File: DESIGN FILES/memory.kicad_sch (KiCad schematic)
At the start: 20 parts, among them J601 TF-15x15, U601 IS42S16160J-6BLI, U602 IS25WP064A-JBLE

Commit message: changes and adding schematic pdf
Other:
- company: Soundsom -> Joël Ucedo
- title: Memory -> MIMXRT1064 MCU Module
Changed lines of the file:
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@@
   (paper "A3")
   (title_block
-    (title "Memory")
-    (date "2023-05-19")
+    (title "MIMXRT1064 MCU Module")
+    (date "2023-05-23")
     (rev "0")
-    (company "Soundsom")
+    (company "Joël Ucedo")
   )
   (junction (at 288.29 102.87) (diameter 0) (color 0 0 0 0)

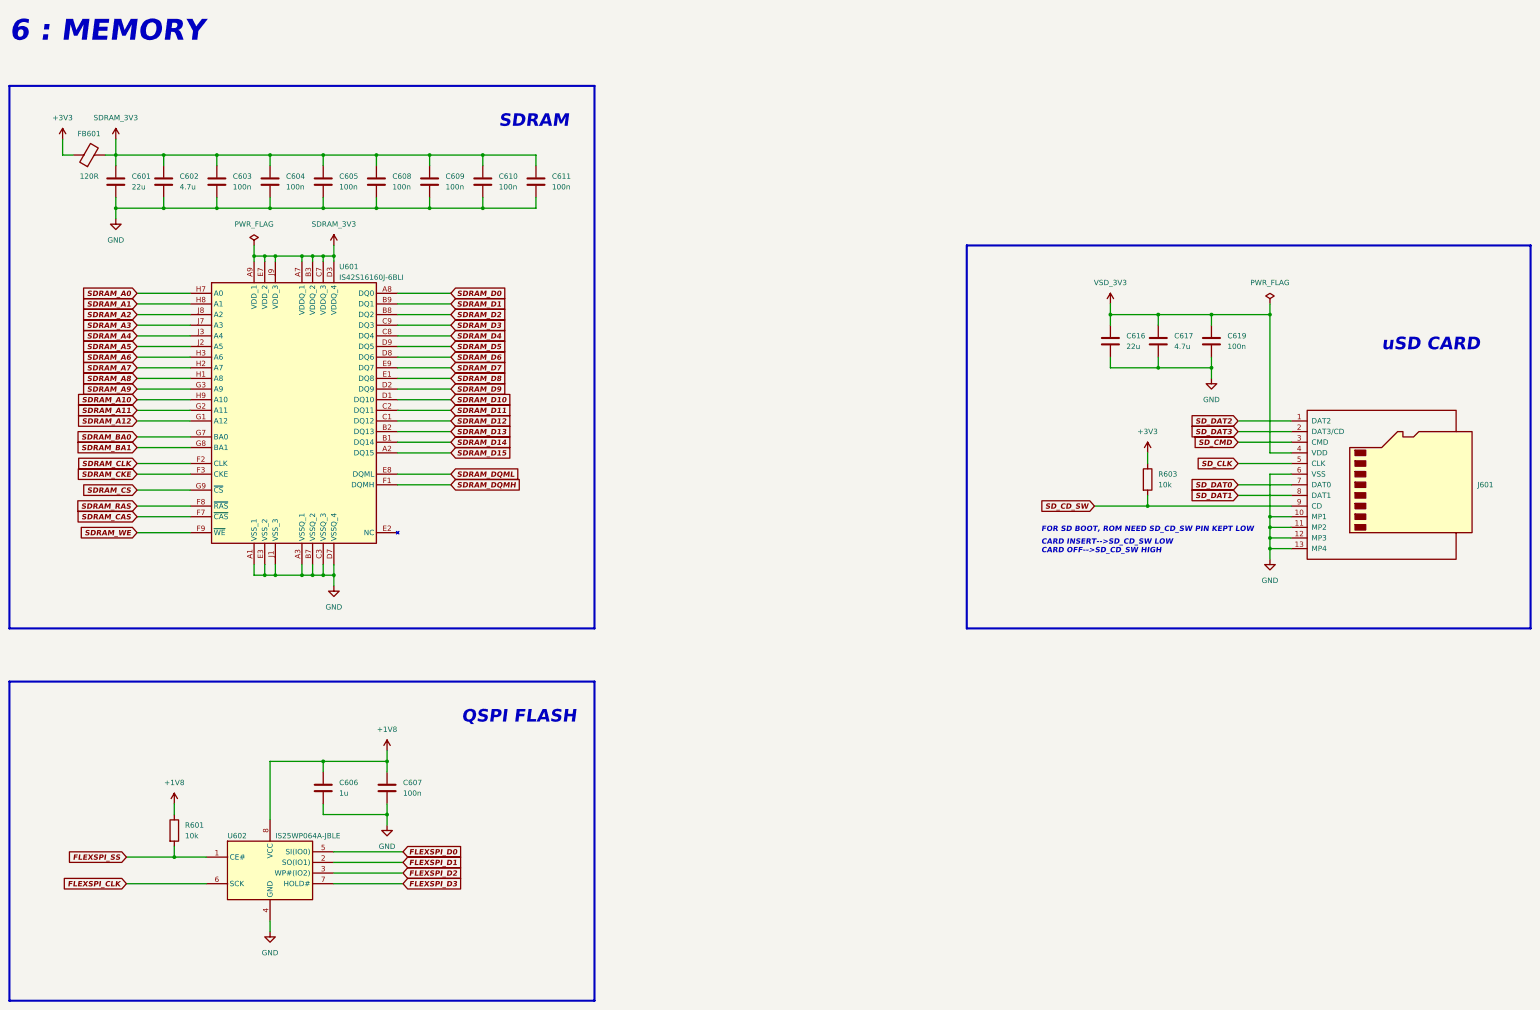
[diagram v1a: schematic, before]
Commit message: updates
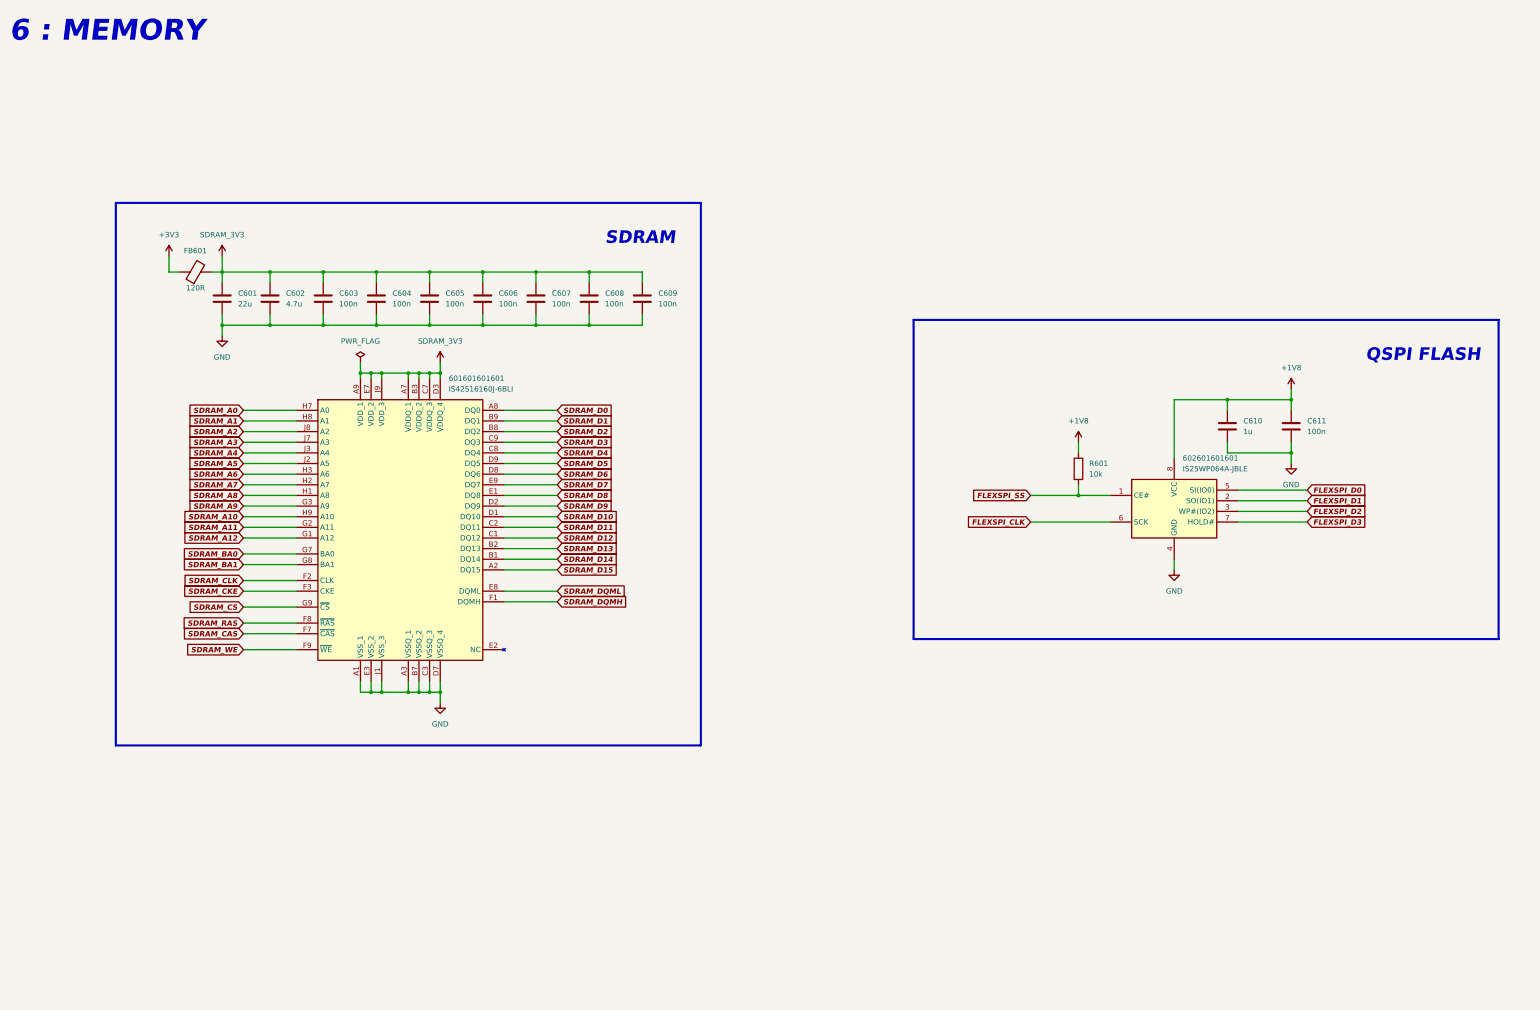
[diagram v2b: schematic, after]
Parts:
- removed C601, C616: 22u, MIMXRT1064 MCU Module:0603_CL10A226MQ8NRNC, symbol MIMXRT1064 MCU Module:CL10A226MQ8NRNC
- removed C602, C617: 4.7u, MIMXRT1064 MCU Module:0402_CL05A475MP5NRNC, symbol MIMXRT1064 MCU Module:CL05A475MP5NRNC
- removed C603, C604, C605, C607, C608, C609, C610, C611, C619: 100n, MIMXRT1064 MCU Module:0402_CL05B104KB54PNC, symbol MIMXRT1064 MCU Module:CL05B104KB54PNC
- removed C606: 1u, MIMXRT1064 MCU Module:0402_CL05A105KA5NQNC, symbol MIMXRT1064 MCU Module:CL05A105KA5NQNC
- removed FB601: 120R, MIMXRT1064 MCU Module:0603_BLM18AG121SN1D, symbol MIMXRT1064 MCU Module:BLM18AG121SN1D
- removed J601: TF-15x15, MIMXRT1064 MCU Module:TF-15x15_smd, symbol MIMXRT1064 MCU Module:TF-15x15
- removed R601, R603: 10k, MIMXRT1064 MCU Module:0402WGF1002TCE, symbol MIMXRT1064 MCU Module:0402WGF1002TCE
- removed U601: IS42S16160J-6BLI, MIMXRT1064 MCU Module:IS42S16160J-6BLI, symbol MIMXRT1064 MCU Module:IS42S16160J-6BLI
- removed U602: IS25WP064A-JBLE, MIMXRT1064 MCU Module:IS25WP064A-JBLE, symbol MIMXRT1064 MCU Module:IS25WP064A-JBLE
- added 601601601601: IS42S16160J-6BLI, MY MEMORY AND STORAGE LIBRARY:IS42S16160J-6BLI, symbol MY MEMORY AND STORAGE LIBRARY:IS42S16160J-6BLI
- added 602601601601: IS25WP064A-JBLE, MY MEMORY AND STORAGE LIBRARY:IS25WP064A-JBLE, symbol MY MEMORY AND STORAGE LIBRARY:IS25WP064A-JBLE
- added C601: 22u, MY CAPACITOR LIBRARY:0603_CL10A226MQ8NRNC, symbol MY CAPACITOR LIBRARY:CL10A226MQ8NRNC
- added C602: 4.7u, MY CAPACITOR LIBRARY:0402_CL05A475MP5NRNC, symbol MY CAPACITOR LIBRARY:CL05A475MP5NRNC
- added C603, C604, C605, C606, C607, C608, C609, C611: 100n, MY CAPACITOR LIBRARY:0402_CL05B104KB54PNC, symbol MY CAPACITOR LIBRARY:CL05B104KB54PNC
- added C610: 1u, MY CAPACITOR LIBRARY:0402_CL05A105KA5NQNC, symbol MY CAPACITOR LIBRARY:CL05A105KA5NQNC
- added FB601: 120R, MY FERRITE BEAD LIBRARY:0603_BLM18AG121SN1D, symbol MY FERRITE BEAD LIBRARY:BLM18AG121SN1D
- added R601: 10k, MY RESISTOR LIBRARY:0402WGF1002TCE, symbol MY RESISTOR LIBRARY:0402WGF1002TCE
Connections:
- net +1V8: now also 602601601601.8 (VCC), C610.1, C611.1, R601.1
- net +3V3: now also FB601.1
- net FLEXSPI_CLK: now also 602601601601.6 (SCK)
- net FLEXSPI_D0: now also 602601601601.5 (SI(IO0))
- net FLEXSPI_D1: now also 602601601601.2 (SO(IO1))
- net FLEXSPI_D2: now also 602601601601.3 (WP#(IO2))
- net FLEXSPI_D3: now also 602601601601.7 (HOLD#)
- net FLEXSPI_SS: now also 602601601601.1 (CE#), R601.2
- net GND: now also 601601601601.A1 (VSS_1), 601601601601.A3 (VSSQ_1), 601601601601.B7 (VSSQ_2), 601601601601.C3 (VSSQ_3), 601601601601.D7 (VSSQ_4), 601601601601.E3 (VSS_2), 601601601601.J1 (VSS_3), 602601601601.4 (GND), C601.2, C602.2, C603.2, C604.2, C605.2, C606.2, C607.2, C608.2, C609.2, C610.2, C611.2
- net SDRAM_3V3: now also 601601601601.A7 (VDDQ_1), 601601601601.A9 (VDD_1), 601601601601.B3 (VDDQ_2), 601601601601.C7 (VDDQ_3), 601601601601.D3 (VDDQ_4), 601601601601.E7 (VDD_2), 601601601601.J9 (VDD_3), C601.1, C602.1, C603.1, C604.1, C605.1, C606.1, C607.1, C608.1, C609.1, FB601.2
- net SDRAM_A0: now also 601601601601.H7 (A0)
- net SDRAM_A1: now also 601601601601.H8 (A1)
- net SDRAM_A10: now also 601601601601.H9 (A10)
- net SDRAM_A11: now also 601601601601.G2 (A11)
- net SDRAM_A12: now also 601601601601.G1 (A12)
- net SDRAM_A2: now also 601601601601.J8 (A2)
- net SDRAM_A3: now also 601601601601.J7 (A3)
- net SDRAM_A4: now also 601601601601.J3 (A4)
- net SDRAM_A5: now also 601601601601.J2 (A5)
- net SDRAM_A6: now also 601601601601.H3 (A6)
- net SDRAM_A7: now also 601601601601.H2 (A7)
- net SDRAM_A8: now also 601601601601.H1 (A8)
- net SDRAM_A9: now also 601601601601.G3 (A9)
- net SDRAM_BA0: now also 601601601601.G7 (BA0)
- net SDRAM_BA1: now also 601601601601.G8 (BA1)
- net SDRAM_CAS: now also 601601601601.F7 (~{CAS})
- net SDRAM_CKE: now also 601601601601.F3 (CKE)
- net SDRAM_CLK: now also 601601601601.F2 (CLK)
- net SDRAM_CS: now also 601601601601.G9 (~{CS})
- net SDRAM_D0: now also 601601601601.A8 (DQ0)
- net SDRAM_D1: now also 601601601601.B9 (DQ1)
- net SDRAM_D10: now also 601601601601.D1 (DQ10)
- net SDRAM_D11: now also 601601601601.C2 (DQ11)
- net SDRAM_D12: now also 601601601601.C1 (DQ12)
- net SDRAM_D13: now also 601601601601.B2 (DQ13)
- net SDRAM_D14: now also 601601601601.B1 (DQ14)
- net SDRAM_D15: now also 601601601601.A2 (DQ15)
- net SDRAM_D2: now also 601601601601.B8 (DQ2)
- net SDRAM_D3: now also 601601601601.C9 (DQ3)
- net SDRAM_D4: now also 601601601601.C8 (DQ4)
- net SDRAM_D5: now also 601601601601.D9 (DQ5)
- net SDRAM_D6: now also 601601601601.D8 (DQ6)
- net SDRAM_D7: now also 601601601601.E9 (DQ7)
- net SDRAM_D8: now also 601601601601.E1 (DQ8)
- net SDRAM_D9: now also 601601601601.D2 (DQ9)
- net SDRAM_DQMH: now also 601601601601.F1 (DQMH)
- net SDRAM_DQML: now also 601601601601.E8 (DQML)
- net SDRAM_RAS: now also 601601601601.F8 (~{RAS})
- net SDRAM_WE: now also 601601601601.F9 (~{WE})
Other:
- note removed: "CARD INSERT-->SD_CD_SW LOW CARD OFF-->SD_CD_SW HIGH"
- note removed: "FOR SD BOOT, ROM NEED SD_CD_SW PIN KEPT LOW"
- note removed: "uSD CARD"
